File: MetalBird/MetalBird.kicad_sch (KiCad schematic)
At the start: 33 parts, among them SW1 SW_Push_Open, U1 STM32F411CEUx, U2 AMS1117-3.3, U3 MPU-6050, Y1 8MHz

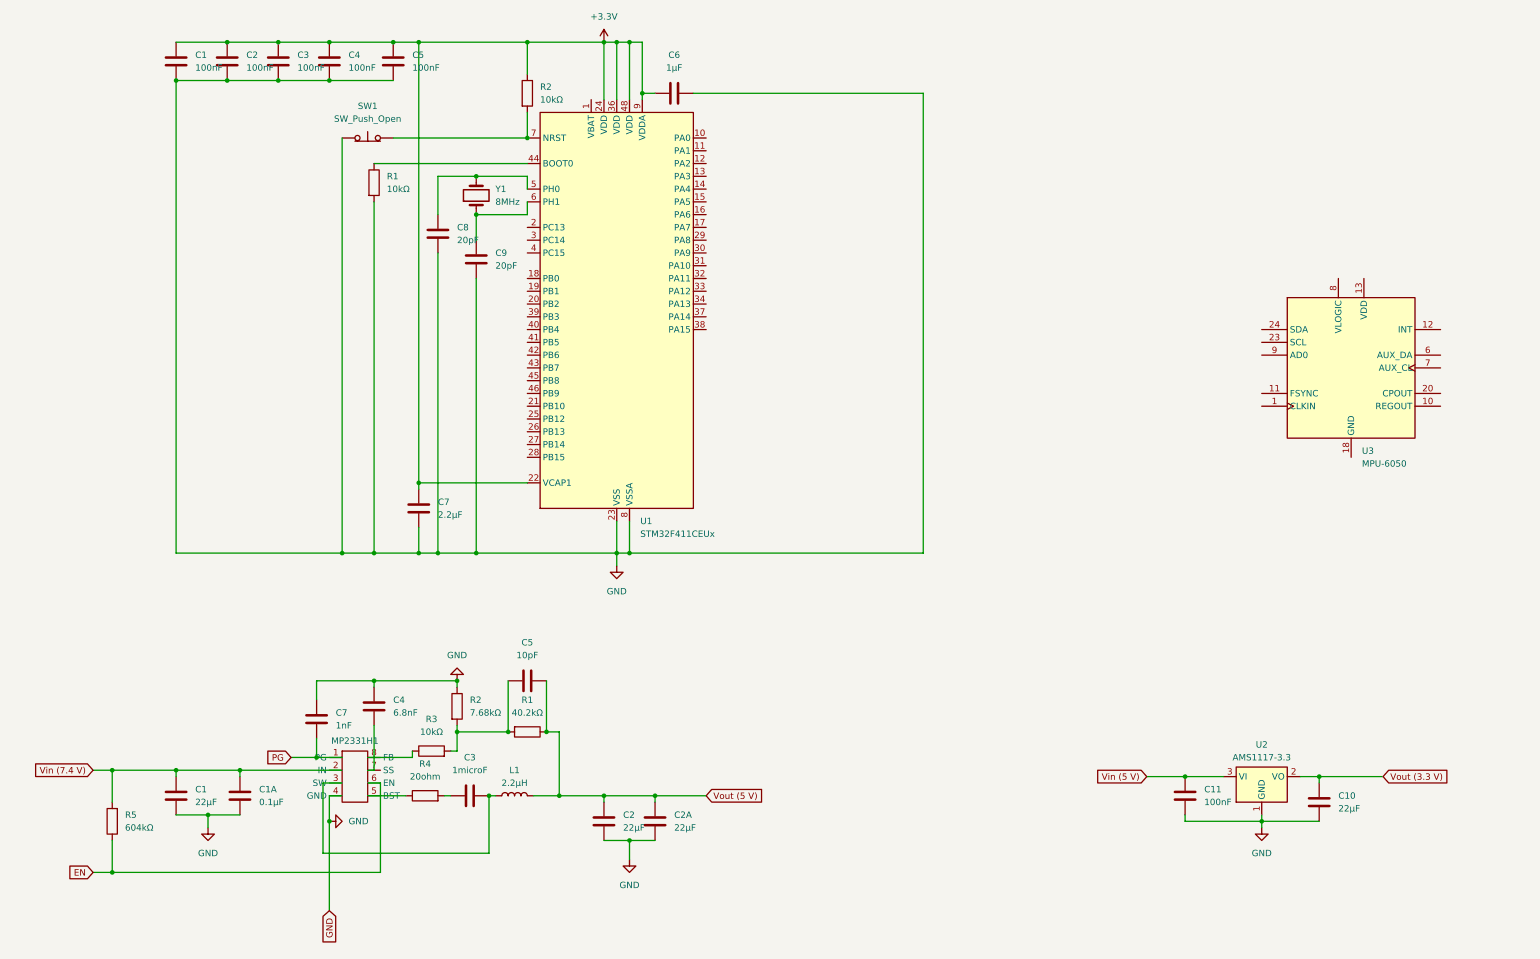
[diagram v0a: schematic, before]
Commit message: IMU Complete
Used MPU-6050 Product specification datasheet for reference
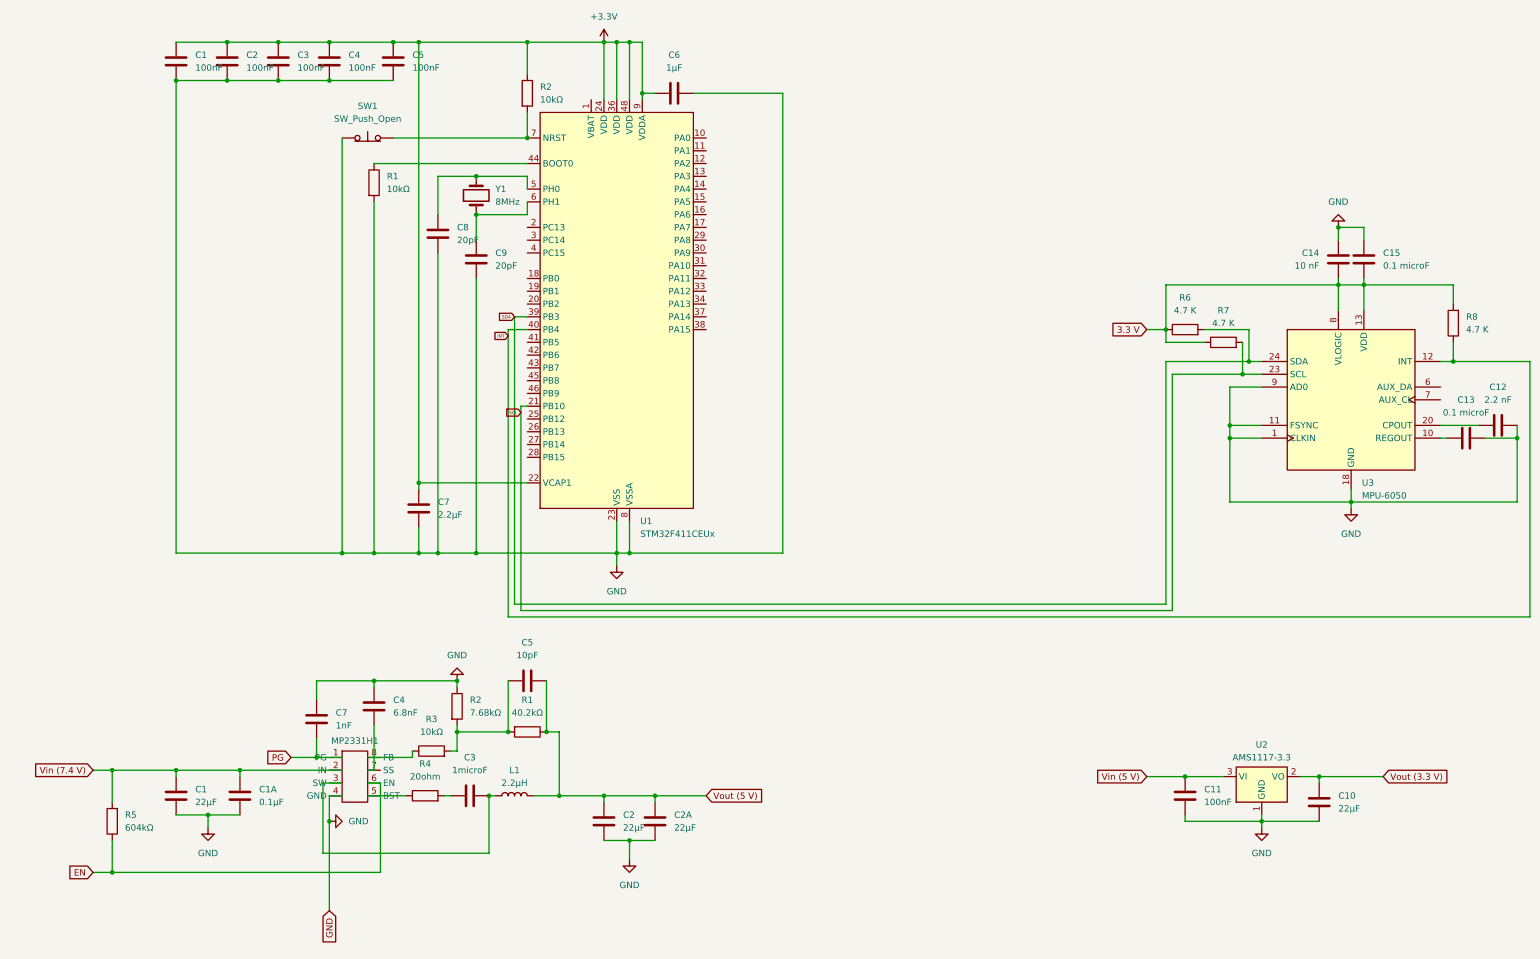
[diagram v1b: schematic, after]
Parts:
- added C12: 2.2 nF, symbol Device:C
- added C13, C15: 0.1 microF, symbol Device:C
- added C14: 10 nF, symbol Device:C
- added R6, R7, R8: 4.7 K, symbol Device:R
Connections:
- net GND: now also U3.1 (CLKIN), U3.11 (FSYNC), U3.18 (GND), U3.9 (AD0), C12.2, C13.2, C14.1, C15.1
- net at U3.10 (REGOUT): now also C13.1
- net INT: now reaches U3.12 (INT)
- net INT: now also U1.40 (PB4), R8.1
- net 3.3 V: now reaches U3.13 (VDD)
- net 3.3 V: now also U3.8 (VLOGIC), C14.2, C15.2, R6.1, R7.1, R8.2
- net at U3.20 (CPOUT): now also C12.1
- net SCL: now reaches U3.23 (SCL)
- net SCL: now also U1.21 (PB10), R7.2
- net SDA: now reaches U3.24 (SDA)
- net SDA: now also U1.39 (PB3), R6.2
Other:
- moved on the sheet: U3
